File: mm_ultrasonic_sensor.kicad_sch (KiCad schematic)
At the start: 0 parts

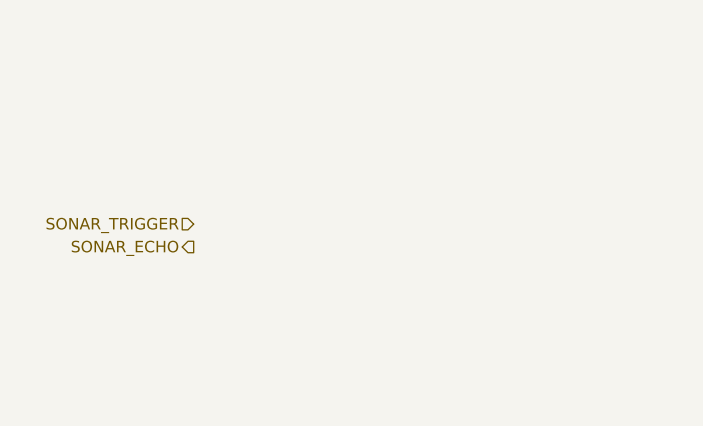
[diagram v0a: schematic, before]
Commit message: fin tp2
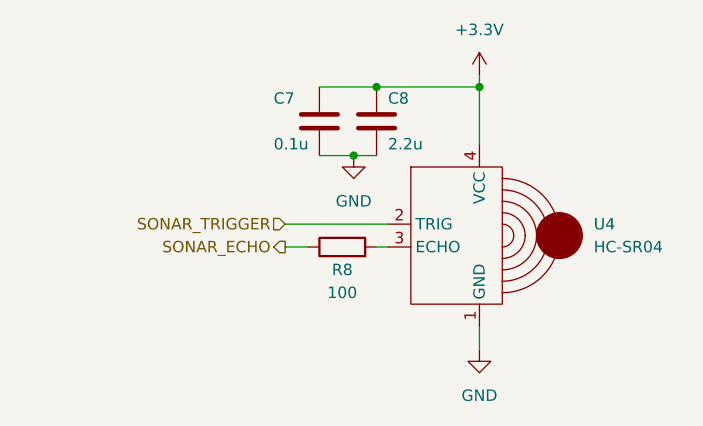
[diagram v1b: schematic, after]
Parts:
- added C7: 0.1u, Capacitor_SMD:C_0603_1608Metric, symbol Device:C
- added C8: 2.2u, Capacitor_SMD:C_0603_1608Metric, symbol Device:C
- added R8: 100, Resistor_SMD:R_0603_1608Metric, symbol Device:R
- added U4: HC-SR04, minimouse:HC-SR04, symbol minimouse:HC-SR04
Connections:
- net SONAR_ECHO: now also R8.1
- net SONAR_TRIGGER: now also U4.2 (TRIG)
- new net: R8.2, U4.3 (ECHO)
- new net +3.3V: C7.1, C8.1, U4.4 (VCC)
- new net GND: C7.2, C8.2, U4.1 (GND)
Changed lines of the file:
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@@
 (kicad_sch (version 20230121) (generator eeschema)
   (paper "A4")
-  (hierarchical_label "SONAR_TRIGGER" (shape input) (at 109.22 88.9 180) (fields_autoplaced)
+  (junction (at 129.54 73.66) (diameter 0) (color 0 0 0 0)
+  )
+  (junction (at 140.97 73.66) (diameter 0) (color 0 0 0 0)
+  )
+  (junction (at 127 81.28) (diameter 0) (color 0 0 0 0)
+  )
+  (wire (pts (xy 129.54 91.44) (xy 130.81 91.44))
+    (stroke (width 0) (type default))
+  )
+  (wire (pts (xy 140.97 100.33) (xy 140.97 102.87))
+    (stroke (width 0) (type default))
+  )
+  (wire (pts (xy 127 81.28) (xy 129.54 81.28))
+    (stroke (width 0) (type default))
+  )
+  (wire (pts (xy 129.54 73.66) (xy 140.97 73.66))
+    (stroke (width 0) (type default))
+  )
+  (wire (pts (xy 123.19 81.28) (xy 127 81.28))
+    (stroke (width 0) (type default))
+  )
+  (wire (pts (xy 119.38 91.44) (xy 121.92 91.44))
+    (stroke (width 0) (type default))
+  )
+  (wire (pts (xy 140.97 72.39) (xy 140.97 73.66))
+    (stroke (width 0) (type default))
+  )
+  (wire (pts (xy 123.19 73.66) (xy 129.54 73.66))
+    (stroke (width 0) (type default))
+  )
+  (wire (pts (xy 140.97 73.66) (xy 140.97 80.01))
+    (stroke (width 0) (type default))
+  )
+  (wire (pts (xy 119.38 88.9) (xy 130.81 88.9))
+    (stroke (width 0) (type default))
+  )
+  (hierarchical_label "SONAR_TRIGGER" (shape input) (at 119.38 88.9 180) (fields_autoplaced)
     (effects (font (size 1.27 1.27)) (justify right))
   )
-  (hierarchical_label "SONAR_ECHO" (shape output) (at 109.22 91.44 180) (fields_autoplaced)
+  (hierarchical_label "SONAR_ECHO" (shape output) (at 119.38 91.44 180) (fields_autoplaced)
     (effects (font (size 1.27 1.27)) (justify right))
   )
+  (symbol (lib_id "Device:R") (at 125.73 91.44 90) (unit 1)
+    (in_bom yes) (on_board yes) (dnp no)
+    (property "Reference" "R8" (at 125.73 93.98 90)
+      (effects (font (size 1.27 1.27)))
+    )
+    (property "Value" "100" (at 125.73 96.52 90)
+      (effects (font (size 1.27 1.27)))
+    )
+    (property "Footprint" "Resistor_SMD:R_0603_1608Metric" (at 125.73 93.218 90)
+      (effects (font (size 1.27 1.27)) hide)
+    )
+    (property "Datasheet" "~" (at 125.73 91.44 0)
+      (effects (font (size 1.27 1.27)) hide)
+    )
+    (pin "1")
+    (pin "2")
+    (instances
+      (project "minimouse"
+        (path "/d8fa4cba-2469-4231-847f-065b6b829f44/b5d7e952-00af-4b6f-924a-ee43c62726d2"
+          (reference "R8") (unit 1)
+        )
+        (path "/d8fa4cba-2469-4231-847f-065b6b829f44/224298a9-7d6e-4a70-a0a5-f2614895ec28"
+          (reference "R26") (unit 1)
+        )
+      )
+    )
+  )
+  (symbol (lib_id "power:+3.3V") (at 140.97 72.39 0) (unit 1)
+    (in_bom yes) (on_board yes) (dnp no) (fields_autoplaced)
+    (property "Reference" "#PWR015" (at 140.97 76.2 0)
+      (effects (font (size 1.27 1.27)) hide)
+    )
+    (property "Value" "+3.3V" (at 140.97 67.31 0)
+      (effects (font (size 1.27 1.27)))
+    )
+    (property "Footprint" "" (at 140.97 72.39 0)
+      (effects (font (size 1.27 1.27)) hide)
+    )
+    (property "Datasheet" "" (at 140.97 72.39 0)
+      (effects (font (size 1.27 1.27)) hide)
+    )
+    (pin "1")
+    (instances
+      (project "minimouse"
+        (path "/d8fa4cba-2469-4231-847f-065b6b829f44/224298a9-7d6e-4a70-a0a5-f2614895ec28"
+          (reference "#PWR015") (unit 1)
+        )
+      )
+    )
+  )
+  (symbol (lib_id "minimouse:HC-SR04") (at 140.97 90.17 0) (unit 1)
+    (in_bom yes) (on_board yes) (dnp no) (fields_autoplaced)
+    (property "Reference" "U4" (at 153.67 88.9 0)
+      (effects (font (size 1.27 1.27)) (justify left))
+    )
+    (property "Value" "HC-SR04" (at 153.67 91.44 0)
+      (effects (font (size 1.27 1.27)) (justify left))
+    )
+    (property "Footprint" "minimouse:HC-SR04" (at 140.97 90.17 0)
+      (effects (font (size 1.27 1.27)) hide)
+    )
+    (property "Datasheet" "" (at 140.97 90.17 0)
+      (effects (font (size 1.27 1.27)) hide)
+    )
+    (pin "1")
+    (pin "4")
+    (pin "3")
+    (pin "2")
+    (instances
+      (project "minimouse"
+        (path "/d8fa4cba-2469-4231-847f-065b6b829f44/224298a9-7d6e-4a70-a0a5-f2614895ec28"
+          (reference "U4") (unit 1)
+        )
+      )
+    )
+  )
+  (symbol (lib_id "power:GND") (at 140.97 102.87 0) (unit 1)
+    (in_bom yes) (on_board yes) (dnp no) (fields_autoplaced)
+    (property "Reference" "#PWR014" (at 140.97 109.22 0)
+      (effects (font (size 1.27 1.27)) hide)
+    )
+    (property "Value" "GND" (at 140.97 107.95 0)
+      (effects (font (size 1.27 1.27)))
+    )
+    (property "Footprint" "" (at 140.97 102.87 0)
+      (effects (font (size 1.27 1.27)) hide)
+    )
+    (property "Datasheet" "" (at 140.97 102.87 0)
+      (effects (font (size 1.27 1.27)) hide)
+    )
+    (pin "1")
+    (instances
+      (project "minimouse"
+        (path "/d8fa4cba-2469-4231-847f-065b6b829f44/224298a9-7d6e-4a70-a0a5-f2614895ec28"
+          (reference "#PWR014") (unit 1)
+        )
+      )
+    )
+  )
+  (symbol (lib_id "Device:C") (at 123.19 77.47 0) (unit 1)
+    (in_bom yes) (on_board yes) (dnp no)
+    (property "Reference" "C7" (at 118.11 74.93 0)
+      (effects (font (size 1.27 1.27)) (justify left))
+    )
+    (property "Value" "0.1u" (at 118.11 80.01 0)
+      (effects (font (size 1.27 1.27)) (justify left))
+    )
+    (property "Footprint" "Capacitor_SMD:C_0603_1608Metric" (at 124.1552 81.28 0)
+      (effects (font (size 1.27 1.27)) hide)
+    )
+    (property "Datasheet" "~" (at 123.19 77.47 0)
+      (effects (font (size 1.27 1.27)) hide)
+    )
+    (pin "1")
+    (pin "2")
+    (instances
+      (project "minimouse"
+        (path "/d8fa4cba-2469-4231-847f-065b6b829f44/0999fad3-9a14-4ede-b729-a71c3dbbdf8e"
+          (reference "C7") (unit 1)
+        )
+        (path "/d8fa4cba-2469-4231-847f-065b6b829f44/224298a9-7d6e-4a70-a0a5-f2614895ec28"
+          (reference "C11") (unit 1)
+        )
+      )
+    )
+  )
+  (symbol (lib_id "Device:C") (at 129.54 77.47 0) (unit 1)
+    (in_bom yes) (on_board yes) (dnp no)
+    (property "Reference" "C8" (at 130.81 74.93 0)
+      (effects (font (size 1.27 1.27)) (justify left))
+    )
+    (property "Value" "2.2u" (at 130.81 80.01 0)
+      (effects (font (size 1.27 1.27)) (justify left))
+    )
+    (property "Footprint" "Capacitor_SMD:C_0603_1608Metric" (at 130.5052 81.28 0)
+      (effects (font (size 1.27 1.27)) hide)
+    )
+    (property "Datasheet" "~" (at 129.54 77.47 0)
+      (effects (font (size 1.27 1.27)) hide)
+    )
+    (pin "1")
+    (pin "2")
+    (instances
+      (project "minimouse"
+        (path "/d8fa4cba-2469-4231-847f-065b6b829f44/0999fad3-9a14-4ede-b729-a71c3dbbdf8e"
+          (reference "C8") (unit 1)
+        )
+        (path "/d8fa4cba-2469-4231-847f-065b6b829f44/7f113667-692a-4f4d-b16f-621d32f3f136"
+          (reference "C17") (unit 1)
+        )
+        (path "/d8fa4cba-2469-4231-847f-065b6b829f44/3975acd0-18ad-47bc-9ce1-d8c4d864aafe"
+          (reference "C18") (unit 1)
+        )
+        (path "/d8fa4cba-2469-4231-847f-065b6b829f44/224298a9-7d6e-4a70-a0a5-f2614895ec28"
+          (reference "C20") (unit 1)
+        )
+      )
+    )
+  )
+  (symbol (lib_id "power:GND") (at 127 81.28 0) (unit 1)
+    (in_bom yes) (on_board yes) (dnp no) (fields_autoplaced)
+    (property "Reference" "#PWR019" (at 127 87.63 0)
+      (effects (font (size 1.27 1.27)) hide)
+    )
+    (property "Value" "GND" (at 127 86.36 0)
+      (effects (font (size 1.27 1.27)))
+    )
+    (property "Footprint" "" (at 127 81.28 0)
+      (effects (font (size 1.27 1.27)) hide)
+    )
+    (property "Datasheet" "" (at 127 81.28 0)
+      (effects (font (size 1.27 1.27)) hide)
+    )
+    (pin "1")
+    (instances
+      (project "minimouse"
+        (path "/d8fa4cba-2469-4231-847f-065b6b829f44/224298a9-7d6e-4a70-a0a5-f2614895ec28"
+          (reference "#PWR019") (unit 1)
+        )
+      )
+    )
+  )
 )
